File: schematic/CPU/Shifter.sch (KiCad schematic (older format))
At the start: 10 parts, among them U19 74LS157, U20 74LS157, U21 74LS157, U22 74LS157, U23 74LS157, U24 74LS157, U25 74LS157, U26 74LS157, U27 74LS157, U28 74LS157

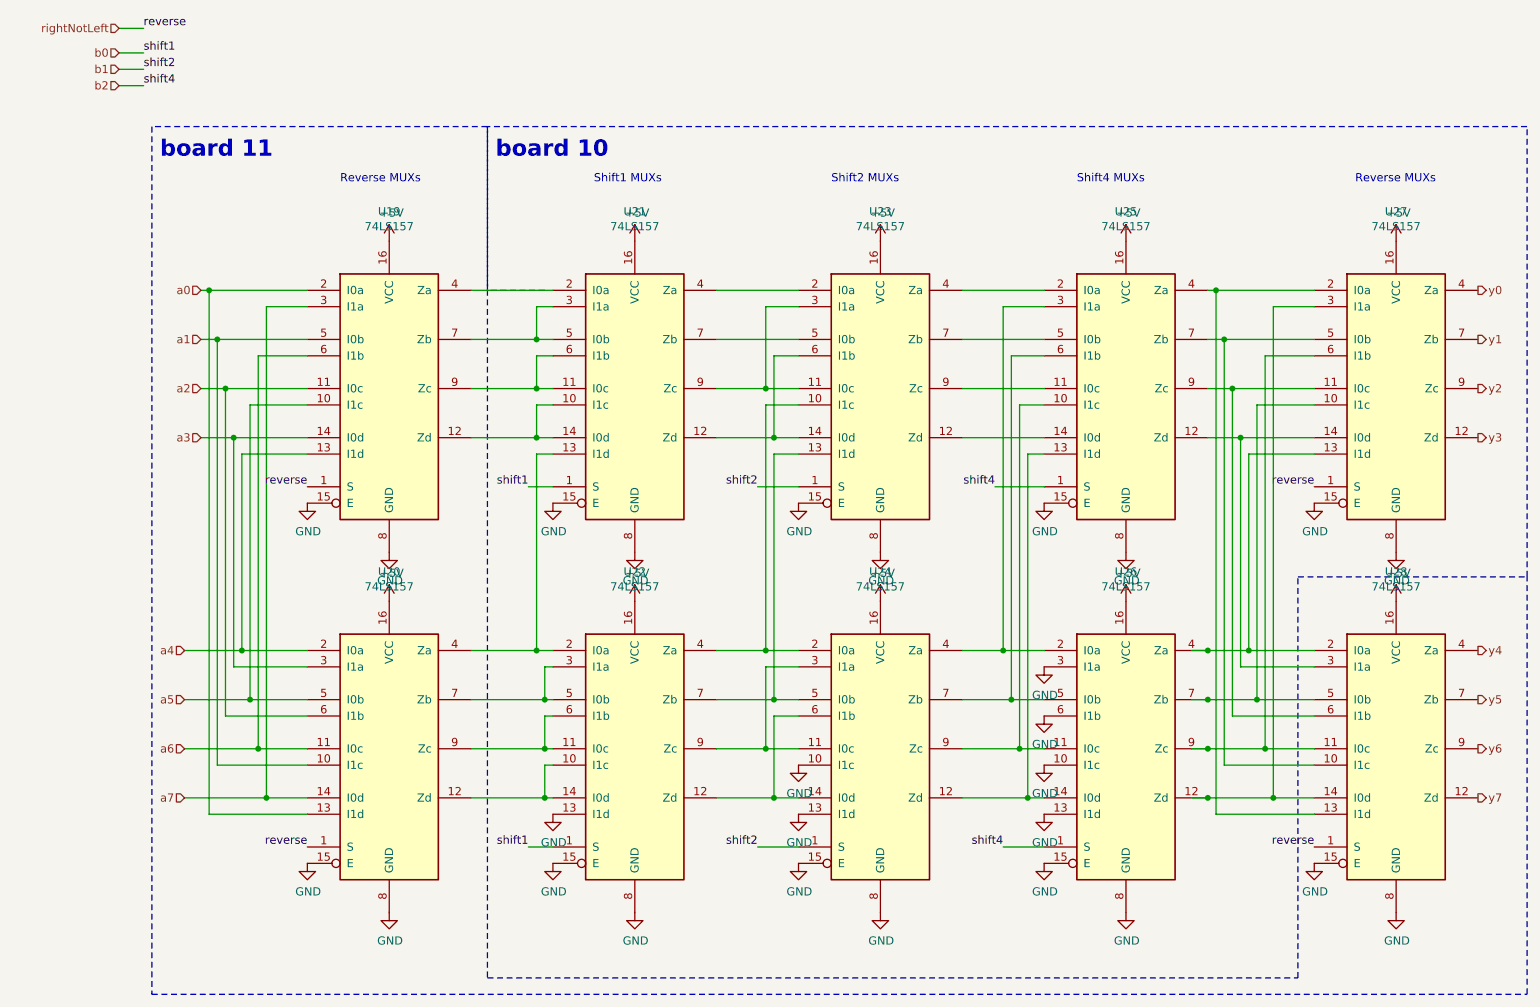
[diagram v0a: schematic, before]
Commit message: schematic with henry
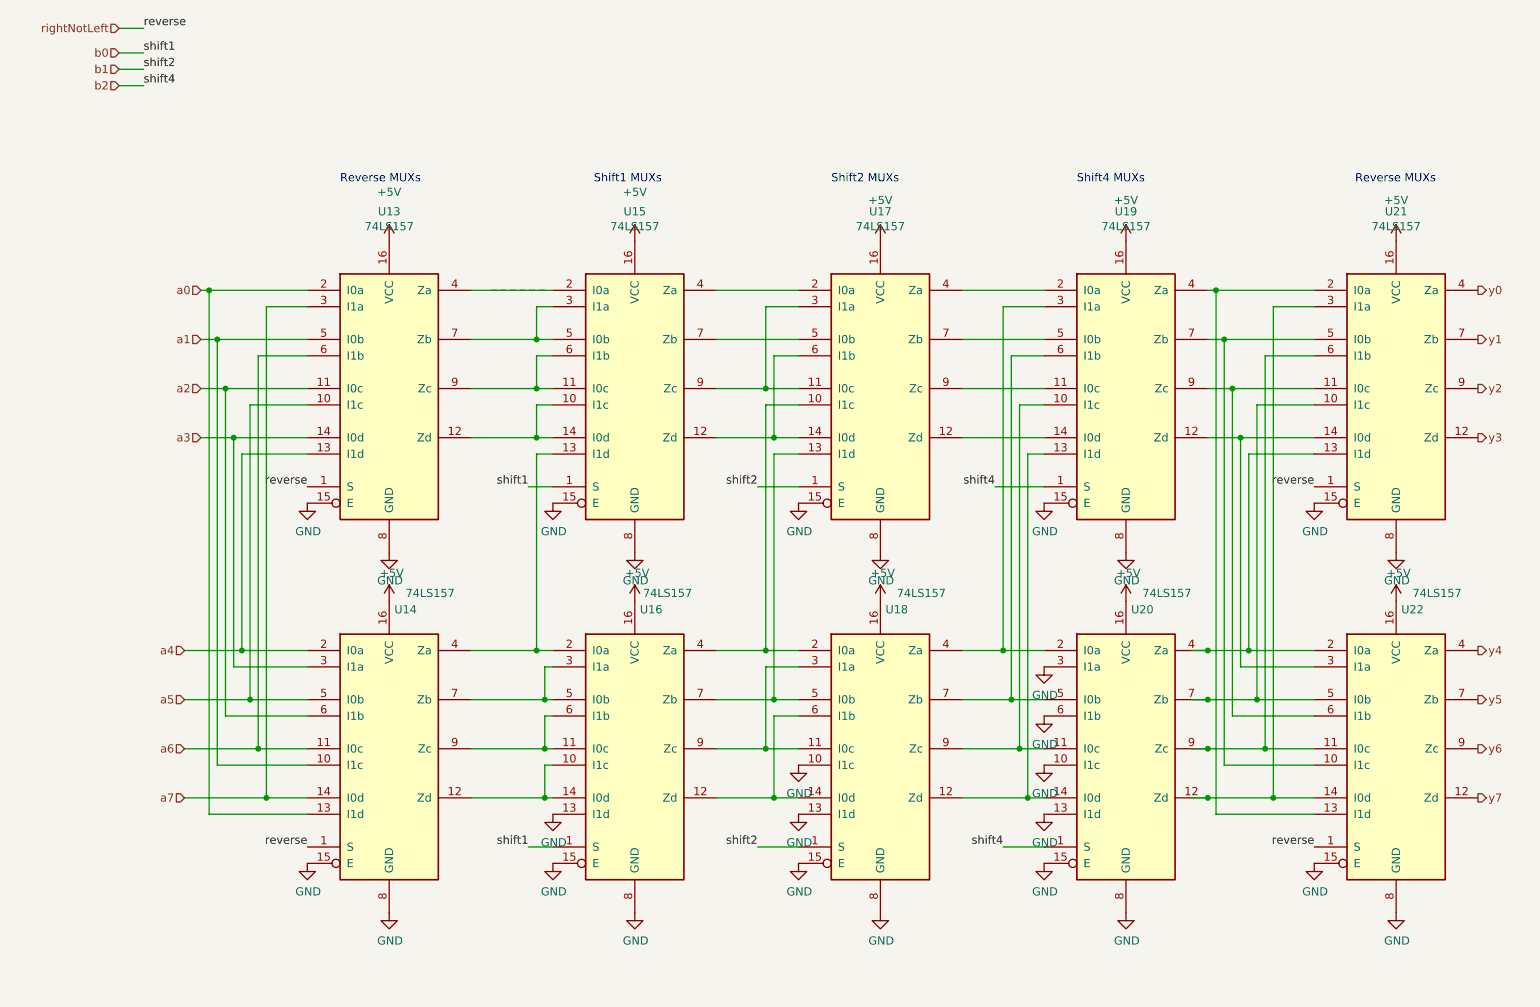
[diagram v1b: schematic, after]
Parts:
- renumbered U19 to U13, U20 to U14, U21 to U15, U22 to U16, U23 to U17, U24 to U18, U25 to U19, U26 to U20, U27 to U21, U28 to U22
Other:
- note removed: "board 10"
- note removed: "board 11\n"
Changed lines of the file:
@@
 $Descr A4 11693 8268
 encoding utf-8
-Sheet 3 17
+Sheet 3 18
 Title ""
 Date ""
@@
 $EndDescr
 $Comp
-L 74xx:74LS157 U19
+L 74xx:74LS157 U13
 U 1 1 6029780F
 P 2650 2800
-F 0 "U19" H 2650 3881 50  0000 C CNN
+F 0 "U13" H 2650 3881 50  0000 C CNN
 F 1 "74LS157" H 2650 3790 50  0000 C CNN
 F 2 "Package_DIP:DIP-16_W7.62mm" H 2650 2800 50  0001 C CNN
@@
 $EndComp
 $Comp
-L 74xx:74LS157 U20
+L 74xx:74LS157 U14
 U 1 1 602993AB
 P 2650 5000
-F 0 "U20" H 2650 6081 50  0000 C CNN
-F 1 "74LS157" H 2650 5990 50  0000 C CNN
+F 0 "U14" H 2750 5850 50  0000 C CNN
+F 1 "74LS157" H 2900 5950 50  0000 C CNN
 F 2 "Package_DIP:DIP-16_W7.62mm" H 2650 5000 50  0001 C CNN
 F 3 "http://www.ti.com/lit/gpn/sn74LS157" H 2650 5000 50  0001 C CNN
@@
 P 2650 1900
 F 0 "#PWR046" H 2650 1750 50  0001 C CNN
-F 1 "+5V" H 2665 2073 50  0000 C CNN
+F 1 "+5V" H 2650 2200 50  0000 C CNN
 F 2 "" H 2650 1900 50  0001 C CNN
 F 3 "" H 2650 1900 50  0001 C CNN
@@
 rightNotLeft
 $Comp
-L 74xx:74LS157 U21
+L 74xx:74LS157 U15
 U 1 1 602A7A35
 P 4150 2800
-F 0 "U21" H 4150 3881 50  0000 C CNN
+F 0 "U15" H 4150 3881 50  0000 C CNN
 F 1 "74LS157" H 4150 3790 50  0000 C CNN
 F 2 "Package_DIP:DIP-16_W7.62mm" H 4150 2800 50  0001 C CNN
@@
 $EndComp
 $Comp
-L 74xx:74LS157 U22
+L 74xx:74LS157 U16
 U 1 1 602A7A3B
 P 4150 5000
-F 0 "U22" H 4150 6081 50  0000 C CNN
-F 1 "74LS157" H 4150 5990 50  0000 C CNN
+F 0 "U16" H 4250 5850 50  0000 C CNN
+F 1 "74LS157" H 4350 5950 50  0000 C CNN
 F 2 "Package_DIP:DIP-16_W7.62mm" H 4150 5000 50  0001 C CNN
 F 3 "http://www.ti.com/lit/gpn/sn74LS157" H 4150 5000 50  0001 C CNN
@@
 P 4150 1900
 F 0 "#PWR053" H 4150 1750 50  0001 C CNN
-F 1 "+5V" H 4165 2073 50  0000 C CNN
+F 1 "+5V" H 4150 2200 50  0000 C CNN
 F 2 "" H 4150 1900 50  0001 C CNN
 F 3 "" H 4150 1900 50  0001 C CNN
@@
 	3550 2500 3150 2500
 $Comp
-L 74xx:74LS157 U23
+L 74xx:74LS157 U17
 U 1 1 602B6E77
 P 5650 2800
-F 0 "U23" H 5650 3881 50  0000 C CNN
+F 0 "U17" H 5650 3881 50  0000 C CNN
 F 1 "74LS157" H 5650 3790 50  0000 C CNN
 F 2 "Package_DIP:DIP-16_W7.62mm" H 5650 2800 50  0001 C CNN
@@
 $EndComp
 $Comp
-L 74xx:74LS157 U24
+L 74xx:74LS157 U18
 U 1 1 602B6E7D
 P 5650 5000
-F 0 "U24" H 5650 6081 50  0000 C CNN
-F 1 "74LS157" H 5650 5990 50  0000 C CNN
+F 0 "U18" H 5750 5850 50  0000 C CNN
+F 1 "74LS157" H 5900 5950 50  0000 C CNN
 F 2 "Package_DIP:DIP-16_W7.62mm" H 5650 5000 50  0001 C CNN
 F 3 "http://www.ti.com/lit/gpn/sn74LS157" H 5650 5000 50  0001 C CNN
@@
 P 5650 1900
 F 0 "#PWR061" H 5650 1750 50  0001 C CNN
-F 1 "+5V" H 5665 2073 50  0000 C CNN
+F 1 "+5V" H 5650 2150 50  0000 C CNN
 F 2 "" H 5650 1900 50  0001 C CNN
 F 3 "" H 5650 1900 50  0001 C CNN
@@
 Shift2 MUXs
 $Comp
-L 74xx:74LS157 U25
+L 74xx:74LS157 U19
 U 1 1 602DB8CC
 P 7150 2800
-F 0 "U25" H 7150 3881 50  0000 C CNN
+F 0 "U19" H 7150 3881 50  0000 C CNN
 F 1 "74LS157" H 7150 3790 50  0000 C CNN
 F 2 "Package_DIP:DIP-16_W7.62mm" H 7150 2800 50  0001 C CNN
@@
 $EndComp
 $Comp
-L 74xx:74LS157 U26
+L 74xx:74LS157 U20
 U 1 1 602DB8D2
 P 7150 5000
-F 0 "U26" H 7150 6081 50  0000 C CNN
-F 1 "74LS157" H 7150 5990 50  0000 C CNN
+F 0 "U20" H 7250 5850 50  0000 C CNN
+F 1 "74LS157" H 7400 5950 50  0000 C CNN
 F 2 "Package_DIP:DIP-16_W7.62mm" H 7150 5000 50  0001 C CNN
 F 3 "http://www.ti.com/lit/gpn/sn74LS157" H 7150 5000 50  0001 C CNN
@@
 P 7150 1900
 F 0 "#PWR071" H 7150 1750 50  0001 C CNN
-F 1 "+5V" H 7165 2073 50  0000 C CNN
+F 1 "+5V" H 7150 2150 50  0000 C CNN
 F 2 "" H 7150 1900 50  0001 C CNN
 F 3 "" H 7150 1900 50  0001 C CNN
@@
 	6350 3400 6650 3400
 $Comp
-L 74xx:74LS157 U27
+L 74xx:74LS157 U21
 U 1 1 6032FFD0
 P 8800 2800
-F 0 "U27" H 8800 3881 50  0000 C CNN
+F 0 "U21" H 8800 3881 50  0000 C CNN
 F 1 "74LS157" H 8800 3790 50  0000 C CNN
 F 2 "Package_DIP:DIP-16_W7.62mm" H 8800 2800 50  0001 C CNN
@@
 $EndComp
 $Comp
-L 74xx:74LS157 U28
+L 74xx:74LS157 U22
 U 1 1 6032FFD6
 P 8800 5000
-F 0 "U28" H 8800 6081 50  0000 C CNN
-F 1 "74LS157" H 8800 5990 50  0000 C CNN
+F 0 "U22" H 8900 5850 50  0000 C CNN
+F 1 "74LS157" H 9050 5950 50  0000 C CNN
 F 2 "Package_DIP:DIP-16_W7.62mm" H 8800 5000 50  0001 C CNN
 F 3 "http://www.ti.com/lit/gpn/sn74LS157" H 8800 5000 50  0001 C CNN
@@
 $EndComp
 $Comp
-L power:GND #PWR079
+L power:GND #PWR080
 U 1 1 6032FFDC
 P 8800 6000
-F 0 "#PWR079" H 8800 5750 50  0001 C CNN
+F 0 "#PWR080" H 8800 5750 50  0001 C CNN
 F 1 "GND" H 8805 5827 50  0000 C CNN
 F 2 "" H 8800 6000 50  0001 C CNN
@@
 $EndComp
 $Comp
-L power:GND #PWR077
+L power:GND #PWR078
 U 1 1 6032FFE8
 P 8800 3800
-F 0 "#PWR077" H 8800 3550 50  0001 C CNN
+F 0 "#PWR078" H 8800 3550 50  0001 C CNN
 F 1 "GND" H 8805 3627 50  0000 C CNN
 F 2 "" H 8800 3800 50  0001 C CNN
@@
 $EndComp
 $Comp
-L power:+5V #PWR078
+L power:+5V #PWR079
 U 1 1 6032FFF4
 P 8800 4100
-F 0 "#PWR078" H 8800 3950 50  0001 C CNN
+F 0 "#PWR079" H 8800 3950 50  0001 C CNN
 F 1 "+5V" H 8815 4273 50  0000 C CNN
 F 2 "" H 8800 4100 50  0001 C CNN
@@
 	7650 5300 8050 5300
 $Comp
-L power:+5V #PWR0108
+L power:+5V #PWR077
 U 1 1 6032FB0C
 P 8800 1900
-F 0 "#PWR0108" H 8800 1750 50  0001 C CNN
-F 1 "+5V" H 8815 2073 50  0000 C CNN
+F 0 "#PWR077" H 8800 1750 50  0001 C CNN
+F 1 "+5V" H 8800 2150 50  0000 C CNN
 F 2 "" H 8800 1900 50  0001 C CNN
 F 3 "" H 8800 1900 50  0001 C CNN
@@
 	1    0    0    -1
 $EndComp
-Wire Notes Line width 12
-	3250 1200 3250 6400
-Wire Notes Line width 12
-	3250 6400 8200 6400
-Wire Notes Line width 12
-	8200 6400 8200 3950
-Wire Notes Line width 12
-	8200 3950 9600 3950
-Wire Notes Line width 12
-	9600 3950 9600 1200
-Wire Notes Line width 12
-	9600 1200 3250 1200
-Text Notes 3300 1400 0    100  ~ 20
-board 10
 Wire Notes Line
 	3600 2200 3250 2200
-Wire Notes Line
-	3250 2200 3250 1200
-Wire Notes Line width 12
-	3250 1200 1200 1200
-Wire Notes Line width 12
-	1200 1200 1200 6500
-Wire Notes Line width 12
-	1200 6500 9600 6500
-Wire Notes Line width 12
-	9600 6500 9600 3950
-Text Notes 1250 1400 0    100  ~ 20
-board 11\n
 $EndSCHEMATC
